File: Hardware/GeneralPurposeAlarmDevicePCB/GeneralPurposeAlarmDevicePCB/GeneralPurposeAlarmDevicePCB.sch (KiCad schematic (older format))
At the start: 42 parts, among them J101 Barrel_Jack_Switch_SMT, J102 22-23-2021, J103 22-23-2021, J105 S04B-XASK-1(LF)(SN), U101 NCP1117ST50T3G, U102 PI_ATMEGA328P-AU-InOrder

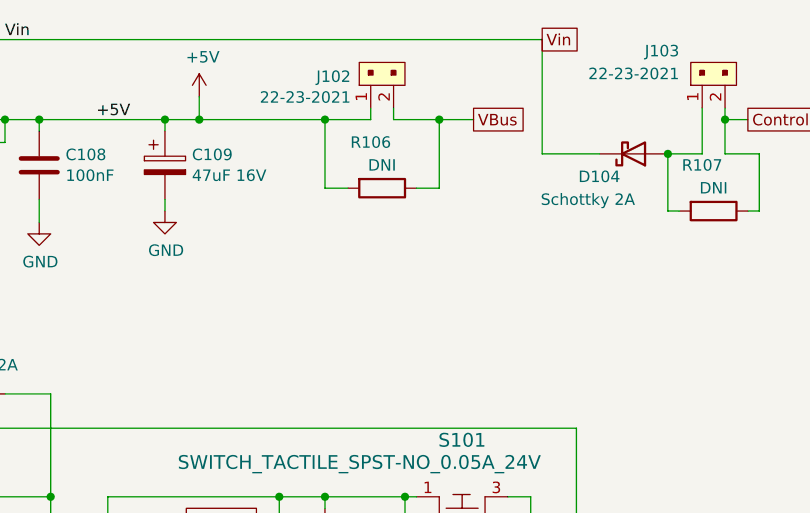
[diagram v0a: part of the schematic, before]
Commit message: Add and LED indicating power on.
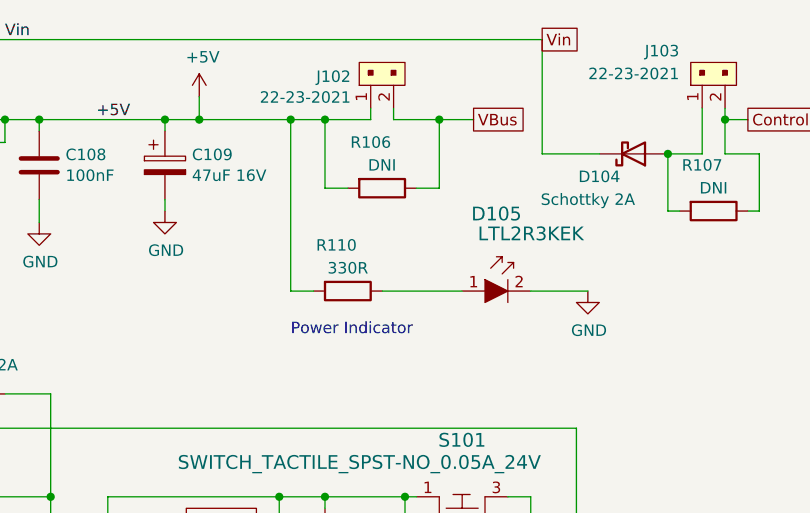
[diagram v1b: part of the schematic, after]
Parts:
- added D105: LTL2R3KEK, GeneralPurposeAlarmDevicePCB:LED_5mm_Radial, symbol dk_LED-Indication-Discrete:LTL2R3KEK
- added R110: 330R, Resistor_SMD:R_0603_1608Metric, symbol Device:R
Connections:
- net +5V: now also R110.2
- net GND: now also D105.2
- new net: D105.1, R110.1
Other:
- note added: "Power Indicator"
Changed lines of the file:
@@
 	2400 950  2500 950
 Wire Wire Line
-	4350 950  4900 950
+	4350 950  4750 950
 $Comp
 L Device:D_Schottky D104
@@
 	1    0    0    -1
 $EndComp
+$Comp
+L dk_LED-Indication-Discrete:LTL2R3KEK D105
+U 1 1 62D73675
+P 5700 1700
+F 0 "D105" H 5650 2037 60  0000 C CNN
+F 1 "LTL2R3KEK" H 5800 1950 60  0000 C CNN
+F 2 "GeneralPurposeAlarmDevicePCB:LED_5mm_Radial" H 5900 1900 60  0001 L CNN
+F 3 "http://optoelectronics.liteon.com/upload/download/DS-20-98-0286/LTL2R3KEK.pdf" H 5900 2000 60  0001 L CNN
+F 4 "160-1682-ND" H 5900 2100 60  0001 L CNN "Digi-Key_PN"
+F 5 "LTL2R3KEK" H 5900 2200 60  0001 L CNN "MPN"
+F 6 "Optoelectronics" H 5900 2300 60  0001 L CNN "Category"
+F 7 "LED Indication - Discrete" H 5900 2400 60  0001 L CNN "Family"
+F 8 "http://optoelectronics.liteon.com/upload/download/DS-20-98-0286/LTL2R3KEK.pdf" H 5900 2500 60  0001 L CNN "DK_Datasheet_Link"
+F 9 "/product-detail/en/lite-on-inc/LTL2R3KEK/160-1682-ND/573572" H 5900 2600 60  0001 L CNN "DK_Detail_Page"
+F 10 "LED RED CLEAR T-1 3/4 T/H" H 5900 2700 60  0001 L CNN "Description"
+F 11 "Lite-On Inc." H 5900 2800 60  0001 L CNN "Manufacturer"
+F 12 "Active" H 5900 2900 60  0001 L CNN "Status"
+	1    5700 1700
+	1    0    0    -1
+$EndComp
+$Comp
+L Device:R R110
+U 1 1 62D74668
+P 5000 1700
+F 0 "R110" V 4800 1650 50  0000 C CNN
+F 1 "330R" V 4900 1700 50  0000 C CNN
+F 2 "Resistor_SMD:R_0603_1608Metric" V 4930 1700 50  0001 C CNN
+F 3 "~" H 5000 1700 50  0001 C CNN
+F 4 "JLCPCB" V 5000 1700 50  0001 C CNN "Distributor 1"
+F 5 "C269711" V 5000 1700 50  0001 C CNN "Distributor 1 PN"
+F 6 "TyoHM" V 5000 1700 50  0001 C CNN "Manufacturer"
+F 7 "RMC06033301%N" V 5000 1700 50  0001 C CNN "MPN"
+F 8 "0.1W ±1% 330Ω 0603 Chip Resistor - Surface Mount ROHS" H 5000 1700 50  0001 C CNN "Description"
+	1    5000 1700
+	0    1    1    0
+$EndComp
+$Comp
+L power:GND #PWR0128
+U 1 1 62D74F16
+P 6050 1700
+F 0 "#PWR0128" H 6050 1450 50  0001 C CNN
+F 1 "GND" H 6055 1527 50  0000 C CNN
+F 2 "" H 6050 1700 50  0001 C CNN
+F 3 "" H 6050 1700 50  0001 C CNN
+	1    6050 1700
+	1    0    0    -1
+$EndComp
+Wire Wire Line
+	6050 1700 5800 1700
+Wire Wire Line
+	4850 1700 4750 1700
+Wire Wire Line
+	4750 1700 4750 950
+Connection ~ 4750 950
+Wire Wire Line
+	4750 950  4900 950
+Text Notes 4750 1900 0    50   ~ 0
+Power Indicator
+Wire Wire Line
+	5500 1700 5150 1700
 $EndSCHEMATC
